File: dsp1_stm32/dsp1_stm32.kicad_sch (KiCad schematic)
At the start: 4 parts

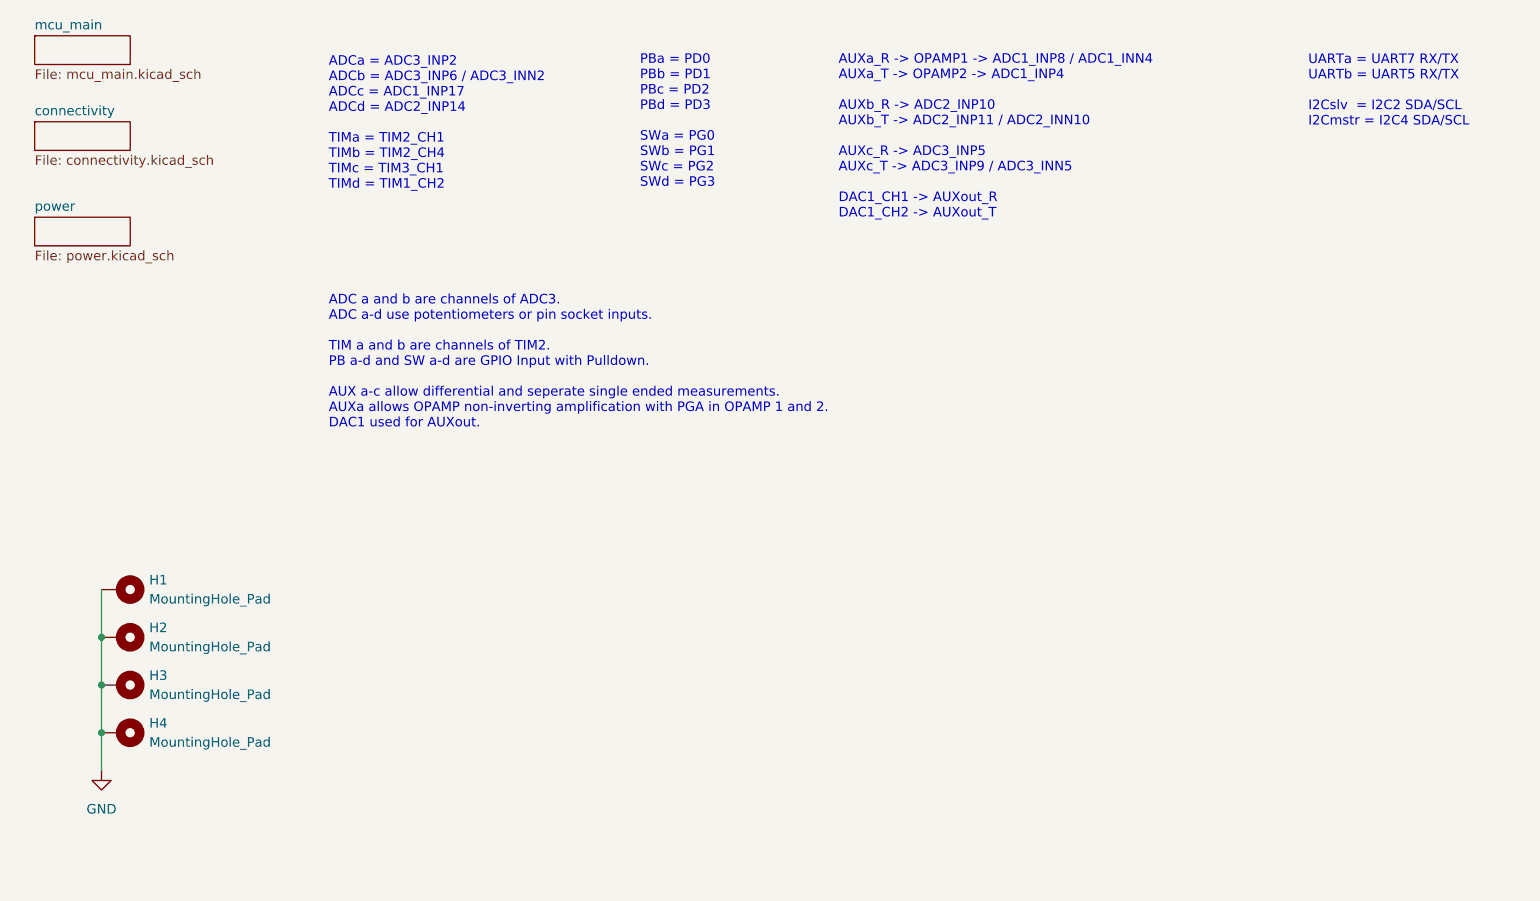
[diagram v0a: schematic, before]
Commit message: PCB dsp v1 done
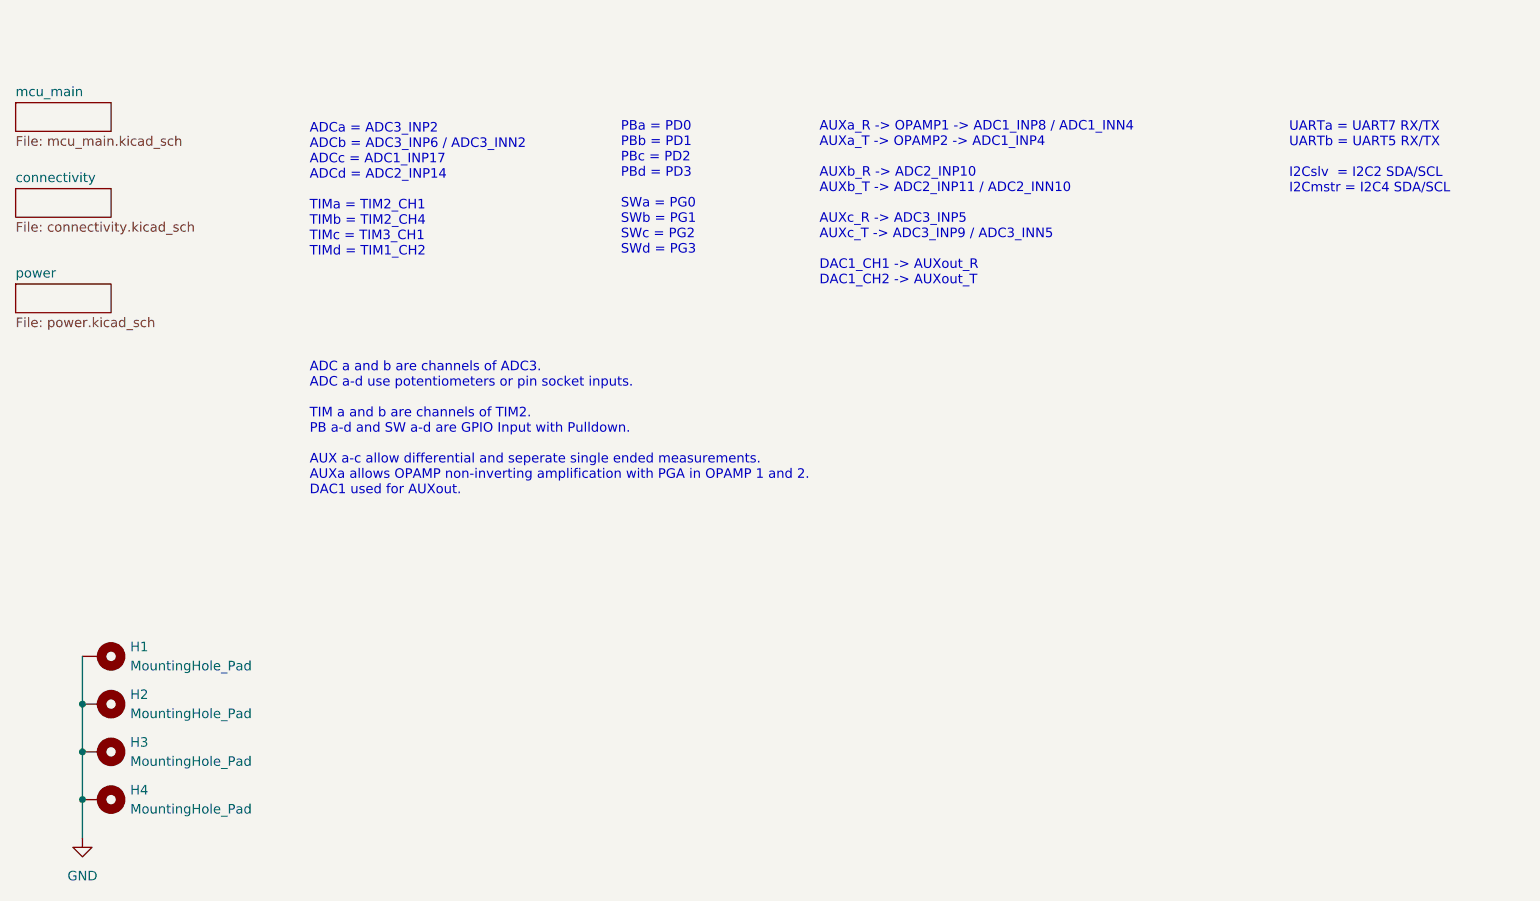
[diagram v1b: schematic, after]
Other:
- moved on the sheet: H1, H2, H3, H4
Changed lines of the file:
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@@
 	(text "PBa = PD0\nPBb = PD1\nPBc = PD2\nPBd = PD3\n\nSWa = PG0\nSWb = PG1\nSWc = PG2\nSWd = PG3"
 		(exclude_from_sim no)
-		(at 116.078 40.64 0)
+		(at 113.538 49.53 0)
 		(effects
 			(font
@@
 	(text "ADCa = ADC3_INP2\nADCb = ADC3_INP6 / ADC3_INN2\nADCc = ADC1_INP17\nADCd = ADC2_INP14\n\nTIMa = TIM2_CH1\nTIMb = TIM2_CH4\nTIMc = TIM3_CH1\nTIMd = TIM1_CH2"
 		(exclude_from_sim no)
-		(at 74.676 40.894 0)
+		(at 72.136 49.784 0)
 		(effects
 			(font
@@
 	(text "ADC a and b are channels of ADC3.\nADC a-d use potentiometers or pin socket inputs.\n\nTIM a and b are channels of TIM2.\nPB a-d and SW a-d are GPIO Input with Pulldown.\n\nAUX a-c allow differential and seperate single ended measurements.\nAUXa allows OPAMP non-inverting amplification with PGA in OPAMP 1 and 2.\nDAC1 used for AUXout."
 		(exclude_from_sim no)
-		(at 74.676 72.644 0)
+		(at 72.136 81.534 0)
 		(effects
 			(font
@@
 	(text "UARTa = UART7 RX/TX\nUARTb = UART5 RX/TX\n\nI2Cslv  = I2C2 SDA/SCL\nI2Cmstr = I2C4 SDA/SCL"
 		(exclude_from_sim no)
-		(at 204.978 36.576 0)
+		(at 202.438 45.466 0)
 		(effects
 			(font
@@
 	(text "AUXa_R -> OPAMP1 -> ADC1_INP8 / ADC1_INN4\nAUXa_T -> OPAMP2 -> ADC1_INP4\n\nAUXb_R -> ADC2_INP10\nAUXb_T -> ADC2_INP11 / ADC2_INN10\n\nAUXc_R -> ADC3_INP5\nAUXc_T -> ADC3_INP9 / ADC3_INN5\n\nDAC1_CH1 -> AUXout_R\nDAC1_CH2 -> AUXout_T"
 		(exclude_from_sim no)
-		(at 142.494 42.672 0)
+		(at 139.954 51.562 0)
 		(effects
 			(font
@@
 	)
 	(junction
-		(at 44.45 109.22)
+		(at 41.91 118.11)
 		(diameter 0)
 		(color 0 0 0 0)
 	)
 	(junction
-		(at 44.45 115.57)
+		(at 41.91 124.46)
 		(diameter 0)
 		(color 0 0 0 0)
 	)
 	(junction
-		(at 44.45 121.92)
+		(at 41.91 130.81)
 		(diameter 0)
 		(color 0 0 0 0)
@@
 	(wire
 		(pts
-			(xy 44.45 109.22) (xy 44.45 115.57)
+			(xy 41.91 118.11) (xy 41.91 124.46)
 		)
 		(stroke
@@
 	(wire
 		(pts
-			(xy 44.45 115.57) (xy 44.45 121.92)
+			(xy 41.91 124.46) (xy 41.91 130.81)
 		)
 		(stroke
@@
 	(wire
 		(pts
-			(xy 44.45 102.87) (xy 44.45 109.22)
+			(xy 41.91 111.76) (xy 41.91 118.11)
 		)
 		(stroke
@@
 	(wire
 		(pts
-			(xy 44.45 121.92) (xy 44.45 127)
+			(xy 41.91 130.81) (xy 41.91 135.89)
 		)
 		(stroke
@@
 	(symbol
 		(lib_id "power:GND")
-		(at 44.45 127 0)
+		(at 41.91 135.89 0)
 		(unit 1)
 		(exclude_from_sim no)
@@
 		(fields_autoplaced yes)
 		(property "Reference" "#PWR01"
-			(at 44.45 133.35 0)
+			(at 41.91 142.24 0)
 			(effects
 				(font
@@
 		)
 		(property "Value" "GND"
-			(at 44.45 132.08 0)
+			(at 41.91 140.97 0)
 			(effects
 				(font
@@
 		)
 		(property "Footprint" ""
-			(at 44.45 127 0)
+			(at 41.91 135.89 0)
 			(effects
 				(font
@@
 		)
 		(property "Datasheet" ""
-			(at 44.45 127 0)
+			(at 41.91 135.89 0)
 			(effects
 				(font
@@
 		)
 		(property "Description" "Power symbol creates a global label with name \"GND\" , ground"
-			(at 44.45 127 0)
+			(at 41.91 135.89 0)
 			(effects
 				(font
@@
 	(symbol
 		(lib_id "Mechanical:MountingHole_Pad")
-		(at 46.99 121.92 270)
+		(at 44.45 130.81 270)
 		(unit 1)
 		(exclude_from_sim no)
@@
 		(fields_autoplaced yes)
 		(property "Reference" "H4"
-			(at 50.8 120.6499 90)
+			(at 48.26 129.5399 90)
 			(effects
 				(font
@@
 		)
 		(property "Value" "MountingHole_Pad"
-			(at 50.8 123.1899 90)
+			(at 48.26 132.0799 90)
 			(effects
 				(font
@@
 		)
 		(property "Footprint" "MountingHole:MountingHole_2.2mm_M2_DIN965_Pad"
-			(at 46.99 121.92 0)
+			(at 44.45 130.81 0)
 			(effects
 				(font
@@
 		)
 		(property "Datasheet" "~"
-			(at 46.99 121.92 0)
+			(at 44.45 130.81 0)
 			(effects
 				(font
@@
 		)
 		(property "Description" "Mounting Hole with connection"
-			(at 46.99 121.92 0)
+			(at 44.45 130.81 0)
 			(effects
 				(font
@@
 	(symbol
 		(lib_id "Mechanical:MountingHole_Pad")
-		(at 46.99 102.87 270)
+		(at 44.45 111.76 270)
 		(unit 1)
 		(exclude_from_sim no)
@@
 		(fields_autoplaced yes)
 		(property "Reference" "H1"
-			(at 50.8 101.5999 90)
+			(at 48.26 110.4899 90)
 			(effects
 				(font
@@
 		)
 		(property "Value" "MountingHole_Pad"
-			(at 50.8 104.1399 90)
+			(at 48.26 113.0299 90)
 			(effects
 				(font
@@
 		)
 		(property "Footprint" "MountingHole:MountingHole_2.2mm_M2_DIN965_Pad"
-			(at 46.99 102.87 0)
+			(at 44.45 111.76 0)
 			(effects
 				(font
@@
 		)
 		(property "Datasheet" "~"
-			(at 46.99 102.87 0)
+			(at 44.45 111.76 0)
 			(effects
 				(font
@@
 		)
 		(property "Description" "Mounting Hole with connection"
-			(at 46.99 102.87 0)
+			(at 44.45 111.76 0)
 			(effects
 				(font
@@
 	(symbol
 		(lib_id "Mechanical:MountingHole_Pad")
-		(at 46.99 115.57 270)
+		(at 44.45 124.46 270)
 		(unit 1)
 		(exclude_from_sim no)
@@
 		(fields_autoplaced yes)
 		(property "Reference" "H3"
-			(at 50.8 114.2999 90)
+			(at 48.26 123.1899 90)
 			(effects
 				(font
@@
 		)
 		(property "Value" "MountingHole_Pad"
-			(at 50.8 116.8399 90)
+			(at 48.26 125.7299 90)
 			(effects
 				(font
@@
 		)
 		(property "Footprint" "MountingHole:MountingHole_2.2mm_M2_DIN965_Pad"
-			(at 46.99 115.57 0)
+			(at 44.45 124.46 0)
 			(effects
 				(font
@@
 		)
 		(property "Datasheet" "~"
-			(at 46.99 115.57 0)
+			(at 44.45 124.46 0)
 			(effects
 				(font
@@
 		)
 		(property "Description" "Mounting Hole with connection"
-			(at 46.99 115.57 0)
+			(at 44.45 124.46 0)
 			(effects
 				(font
@@
 	(symbol
 		(lib_id "Mechanical:MountingHole_Pad")
-		(at 46.99 109.22 270)
+		(at 44.45 118.11 270)
 		(unit 1)
 		(exclude_from_sim no)
@@
 		(fields_autoplaced yes)
 		(property "Reference" "H2"
-			(at 50.8 107.9499 90)
+			(at 48.26 116.8399 90)
 			(effects
 				(font
@@
 		)
 		(property "Value" "MountingHole_Pad"
-			(at 50.8 110.4899 90)
+			(at 48.26 119.3799 90)
 			(effects
 				(font
@@
 		)
 		(property "Footprint" "MountingHole:MountingHole_2.2mm_M2_DIN965_Pad"
-			(at 46.99 109.22 0)
+			(at 44.45 118.11 0)
 			(effects
 				(font
@@
 		)
 		(property "Datasheet" "~"
-			(at 46.99 109.22 0)
+			(at 44.45 118.11 0)
 			(effects
 				(font
@@
 		)
 		(property "Description" "Mounting Hole with connection"
-			(at 46.99 109.22 0)
+			(at 44.45 118.11 0)
 			(effects
 				(font
@@
 	)
 	(sheet
-		(at 35.56 40.64)
+		(at 33.02 49.53)
 		(size 12.7 3.81)
 		(exclude_from_sim no)
@@
 		)
 		(property "Sheetname" "connectivity"
-			(at 35.56 39.9284 0)
+			(at 33.02 48.8184 0)
 			(effects
 				(font
@@
 		)
 		(property "Sheetfile" "connectivity.kicad_sch"
-			(at 35.56 45.0346 0)
+			(at 33.02 53.9246 0)
 			(effects
 				(font
@@
 	)
 	(sheet
-		(at 35.56 53.34)
+		(at 33.02 62.23)
 		(size 12.7 3.81)
 		(exclude_from_sim no)
@@
 		)
 		(property "Sheetname" "power"
-			(at 35.56 52.6284 0)
+			(at 33.02 61.5184 0)
 			(effects
 				(font
@@
 		)
 		(property "Sheetfile" "power.kicad_sch"
-			(at 35.56 57.7346 0)
+			(at 33.02 66.6246 0)
 			(effects
 				(font
@@
 	)
 	(sheet
-		(at 35.56 29.21)
+		(at 33.02 38.1)
 		(size 12.7 3.81)
 		(exclude_from_sim no)
@@
 		)
 		(property "Sheetname" "mcu_main"
-			(at 35.56 28.4984 0)
+			(at 33.02 37.3884 0)
 			(effects
 				(font
@@
 		)
 		(property "Sheetfile" "mcu_main.kicad_sch"
-			(at 35.56 33.6046 0)
-			(effects
-				(font
+			(at 33.02 42.4946 0)
+			(effects
+				(font
